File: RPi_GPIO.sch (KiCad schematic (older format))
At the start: 1 part, among them J2 RPi_GPIO

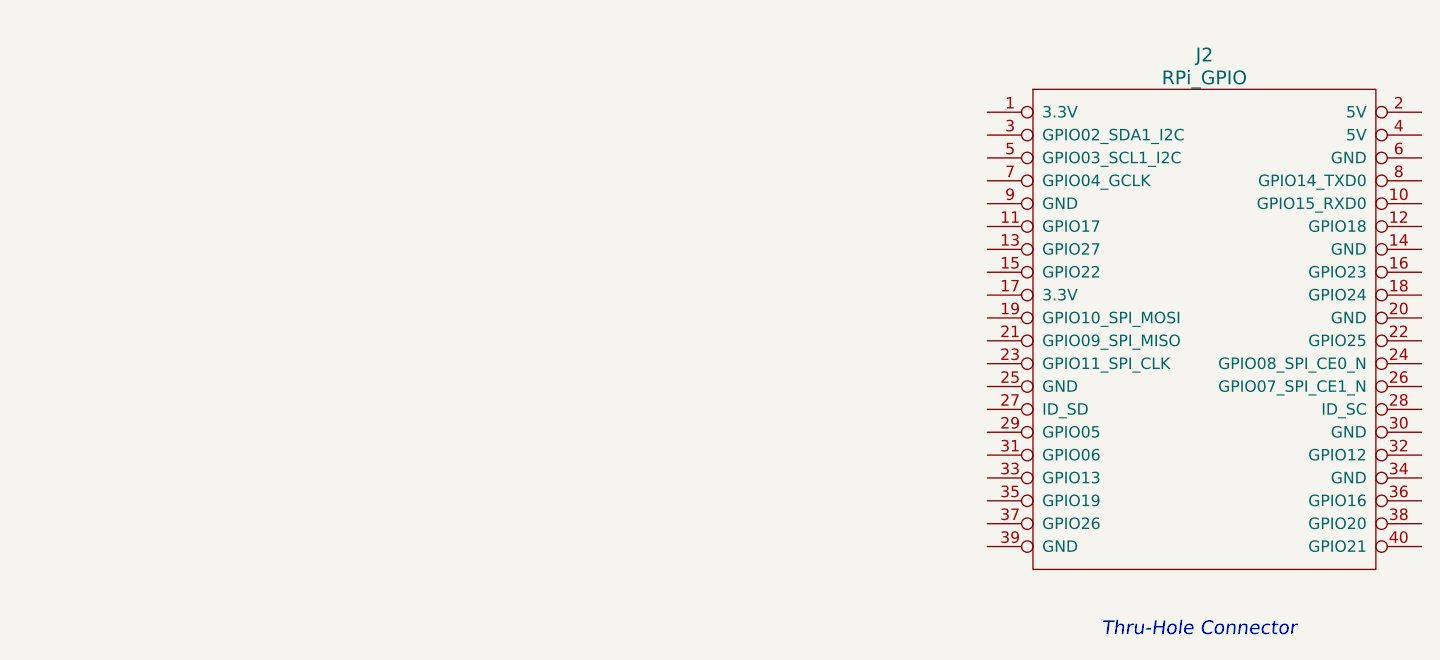
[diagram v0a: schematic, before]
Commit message: Taped out
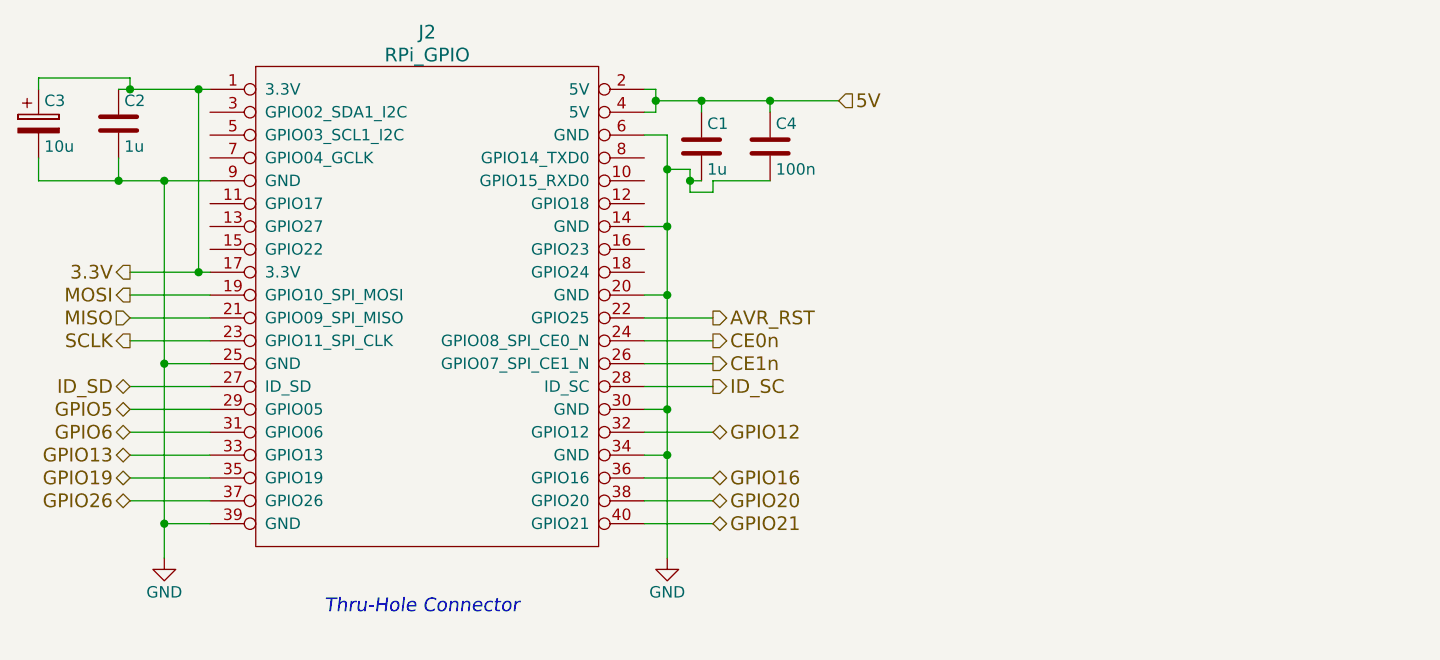
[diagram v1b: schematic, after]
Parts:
- added C1, C2: 1u, Capacitors_SMD:C_0603_HandSoldering, symbol C
- added C3: 10u, Capacitors_Tantalum_SMD:TantalC_SizeA_EIA-3216_HandSoldering, symbol CP
- added C4: 100n, Capacitors_SMD:C_0603_HandSoldering, symbol C
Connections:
- net 3.3V: now reaches J2.1 (3.3V)
- net 3.3V: now also J2.17 (3.3V), C2.1, C3.1
- net GND: now reaches J2.14 (GND)
- net GND: now also J2.20 (GND), J2.25 (GND), J2.30 (GND), J2.34 (GND), J2.39 (GND), J2.6 (GND), J2.9 (GND), C1.2, C2.2, C3.2, C4.2
- net MOSI: now reaches J2.19 (GPIO10_SPI_MOSI)
- net 5V: now reaches J2.2 (5V)
- net 5V: now also J2.4 (5V), C1.1, C4.1
- net MISO: now reaches J2.21 (GPIO09_SPI_MISO)
- net AVR_RST: now reaches J2.22 (GPIO25)
- net SCLK: now reaches J2.23 (GPIO11_SPI_CLK)
- net CE0n: now reaches J2.24 (GPIO08_SPI_CE0_N)
- net CE1n: now reaches J2.26 (GPIO07_SPI_CE1_N)
- net ID_SD: now reaches J2.27 (ID_SD)
- net ID_SC: now reaches J2.28 (ID_SC)
- net GPIO5: now reaches J2.29 (GPIO05)
- net GPIO6: now reaches J2.31 (GPIO06)
- net GPIO12: now reaches J2.32 (GPIO12)
- net GPIO13: now reaches J2.33 (GPIO13)
- net GPIO19: now reaches J2.35 (GPIO19)
- net GPIO16: now reaches J2.36 (GPIO16)
- net GPIO26: now reaches J2.37 (GPIO26)
- net GPIO20: now reaches J2.38 (GPIO20)
- net GPIO21: now reaches J2.40 (GPIO21)
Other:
- moved on the sheet: J2
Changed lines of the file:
@@
 LIBS:contrib
 LIBS:valves
+LIBS:MP1496
 LIBS:RPi_Hat-cache
 EELAYER 25 0
@@
 $Descr A4 11693 8268
 encoding utf-8
-Sheet 2 2
+Sheet 2 3
 Title ""
 Date ""
@@
 L RPi_GPIO J2
 U 1 1 5516AE26
-P 7500 2700
-F 0 "J2" H 8250 2950 60  0000 C CNN
-F 1 "RPi_GPIO" H 8250 2850 60  0000 C CNN
-F 2 "RPi_Hat:Pin_Header_Straight_2x20" H 7500 2700 60  0001 C CNN
-F 3 "" H 7500 2700 60  0000 C CNN
-	1    7500 2700
-	1    0    0    -1
-$EndComp
-Text Notes 7800 5000 0    60   Italic 0
+P 4100 2600
+F 0 "J2" H 4850 2850 60  0000 C CNN
+F 1 "RPi_GPIO" H 4850 2750 60  0000 C CNN
+F 2 "RPi_Hat:Pin_Header_Straight_2x20" H 4100 2600 60  0001 C CNN
+F 3 "" H 4100 2600 60  0000 C CNN
+	1    4100 2600
+	1    0    0    -1
+$EndComp
+Text Notes 4400 4900 0    60   Italic 0
 Thru-Hole Connector
+Text HLabel 6650 2650 2    60   Input ~ 0
+5V
+Wire Wire Line
+	5850 2650 6650 2650
+Wire Wire Line
+	5850 2600 5850 2700
+Wire Wire Line
+	5850 2700 5800 2700
+Wire Wire Line
+	5850 2600 5800 2600
+Connection ~ 5850 2650
+$Comp
+L GND #PWR016
+U 1 1 553C1436
+P 5900 4650
+F 0 "#PWR016" H 5900 4400 50  0001 C CNN
+F 1 "GND" H 5900 4500 50  0000 C CNN
+F 2 "" H 5900 4650 60  0000 C CNN
+F 3 "" H 5900 4650 60  0000 C CNN
+	1    5900 4650
+	1    0    0    -1
+$EndComp
+Wire Wire Line
+	5900 2800 5900 4650
+Wire Wire Line
+	5900 4200 5800 4200
+Wire Wire Line
+	5900 4000 5800 4000
+Connection ~ 5900 4200
+Wire Wire Line
+	5900 3500 5800 3500
+Connection ~ 5900 4000
+Wire Wire Line
+	5800 3200 5900 3200
+Connection ~ 5900 3500
+Wire Wire Line
+	5900 2800 5800 2800
+Connection ~ 5900 3200
+$Comp
+L GND #PWR017
+U 1 1 553C1490
+P 3700 4650
+F 0 "#PWR017" H 3700 4400 50  0001 C CNN
+F 1 "GND" H 3700 4500 50  0000 C CNN
+F 2 "" H 3700 4650 60  0000 C CNN
+F 3 "" H 3700 4650 60  0000 C CNN
+	1    3700 4650
+	1    0    0    -1
+$EndComp
+Wire Wire Line
+	3700 3000 3700 4650
+Wire Wire Line
+	3700 4500 3900 4500
+Wire Wire Line
+	3700 3800 3900 3800
+Connection ~ 3700 4500
+Wire Wire Line
+	3150 3000 3900 3000
+Connection ~ 3700 3800
+Text HLabel 3550 3500 0    60   Output ~ 0
+MOSI
+Wire Wire Line
+	3550 3500 3900 3500
+Text HLabel 3550 3600 0    60   Input ~ 0
+MISO
+Wire Wire Line
+	3550 3600 3900 3600
+Text HLabel 3550 3700 0    60   Output ~ 0
+SCLK
+Wire Wire Line
+	3550 3700 3900 3700
+Text HLabel 3550 3400 0    60   Output ~ 0
+3.3V
+Wire Wire Line
+	3550 3400 3900 3400
+Wire Wire Line
+	3850 3400 3850 2600
+Wire Wire Line
+	3500 2600 3900 2600
+Connection ~ 3850 3400
+Text HLabel 6100 3700 2    60   Output ~ 0
+CE0n
+Wire Wire Line
+	6100 3700 5800 3700
+Text HLabel 6100 3800 2    60   Output ~ 0
+CE1n
+Wire Wire Line
+	6100 3800 5800 3800
+Text HLabel 6100 3600 2    60   Output ~ 0
+AVR_RST
+Wire Wire Line
+	5800 3600 6100 3600
+Text HLabel 6100 3900 2    60   Output ~ 0
+ID_SC
+Wire Wire Line
+	6100 3900 5800 3900
+Text HLabel 3550 3900 0    60   BiDi ~ 0
+ID_SD
+Wire Wire Line
+	3550 3900 3900 3900
+Text HLabel 3550 4000 0    60   BiDi ~ 0
+GPIO5
+Text HLabel 3550 4100 0    60   BiDi ~ 0
+GPIO6
+Text HLabel 3550 4200 0    60   BiDi ~ 0
+GPIO13
+Text HLabel 3550 4300 0    60   BiDi ~ 0
+GPIO19
+Text HLabel 3550 4400 0    60   BiDi ~ 0
+GPIO26
+Wire Wire Line
+	3550 4000 3900 4000
+Wire Wire Line
+	3900 4100 3550 4100
+Wire Wire Line
+	3550 4200 3900 4200
+Wire Wire Line
+	3900 4300 3550 4300
+Wire Wire Line
+	3550 4400 3900 4400
+Text HLabel 6100 4100 2    60   BiDi ~ 0
+GPIO12
+Text HLabel 6100 4300 2    60   BiDi ~ 0
+GPIO16
+Text HLabel 6100 4400 2    60   BiDi ~ 0
+GPIO20
+Text HLabel 6100 4500 2    60   BiDi ~ 0
+GPIO21
+Wire Wire Line
+	5800 4100 6100 4100
+Wire Wire Line
+	5800 4300 6100 4300
+Wire Wire Line
+	5800 4400 6100 4400
+Wire Wire Line
+	5800 4500 6100 4500
+$Comp
+L C C1
+U 1 1 554B2BA7
+P 6050 2850
+F 0 "C1" H 6075 2950 50  0000 L CNN
+F 1 "1u" H 6075 2750 50  0000 L CNN
+F 2 "Capacitors_SMD:C_0603_HandSoldering" H 6088 2700 30  0001 C CNN
+F 3 "" H 6050 2850 60  0000 C CNN
+	1    6050 2850
+	1    0    0    -1
+$EndComp
+Wire Wire Line
+	6050 2650 6050 2700
+Connection ~ 6050 2650
+Wire Wire Line
+	6050 3000 6000 3000
+Wire Wire Line
+	6000 2950 6000 3050
+Wire Wire Line
+	6000 2950 5900 2950
+Connection ~ 5900 2950
+$Comp
+L C C2
+U 1 1 554B32A8
+P 3500 2750
+F 0 "C2" H 3525 2850 50  0000 L CNN
+F 1 "1u" H 3525 2650 50  0000 L CNN
+F 2 "Capacitors_SMD:C_0603_HandSoldering" H 3538 2600 30  0001 C CNN
+F 3 "" H 3500 2750 60  0000 C CNN
+	1    3500 2750
+	1    0    0    -1
+$EndComp
+Connection ~ 3850 2600
+Wire Wire Line
+	3500 2900 3500 3000
+Connection ~ 3700 3000
+$Comp
+L C C4
+U 1 1 555A9EB5
+P 6350 2850
+F 0 "C4" H 6375 2950 50  0000 L CNN
+F 1 "100n" H 6375 2750 50  0000 L CNN
+F 2 "Capacitors_SMD:C_0603_HandSoldering" H 6388 2700 30  0001 C CNN
+F 3 "" H 6350 2850 60  0000 C CNN
+	1    6350 2850
+	1    0    0    -1
+$EndComp
+Wire Wire Line
+	6350 2700 6350 2650
+Connection ~ 6350 2650
+Wire Wire Line
+	6350 3000 6100 3000
+Wire Wire Line
+	6100 3000 6100 3050
+Wire Wire Line
+	6100 3050 6000 3050
+Connection ~ 6000 3000
+$Comp
+L CP C3
+U 1 1 555A9FAB
+P 3150 2750
+F 0 "C3" H 3175 2850 50  0000 L CNN
+F 1 "10u" H 3175 2650 50  0000 L CNN
+F 2 "Capacitors_Tantalum_SMD:TantalC_SizeA_EIA-3216_HandSoldering" H 3188 2600 30  0001 C CNN
+F 3 "" H 3150 2750 60  0000 C CNN
+	1    3150 2750
+	1    0    0    -1
+$EndComp
+Wire Wire Line
+	3150 2600 3150 2550
+Wire Wire Line
+	3150 2550 3550 2550
+Wire Wire Line
+	3550 2550 3550 2600
+Connection ~ 3550 2600
+Wire Wire Line
+	3150 2900 3150 3000
+Connection ~ 3500 3000
 $EndSCHEMATC
